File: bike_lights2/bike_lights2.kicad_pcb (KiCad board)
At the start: 2 copper layers, 36 x 18 mm, 36 parts, among them J2 LED, J3 B+, P1 USB_C_Plug_USB2.0, SW1 TL49, U1 TL431DBZ, U3 MIC2289, U4 MCP6002-xMS, U5 MCP73831-2-ADI/OT

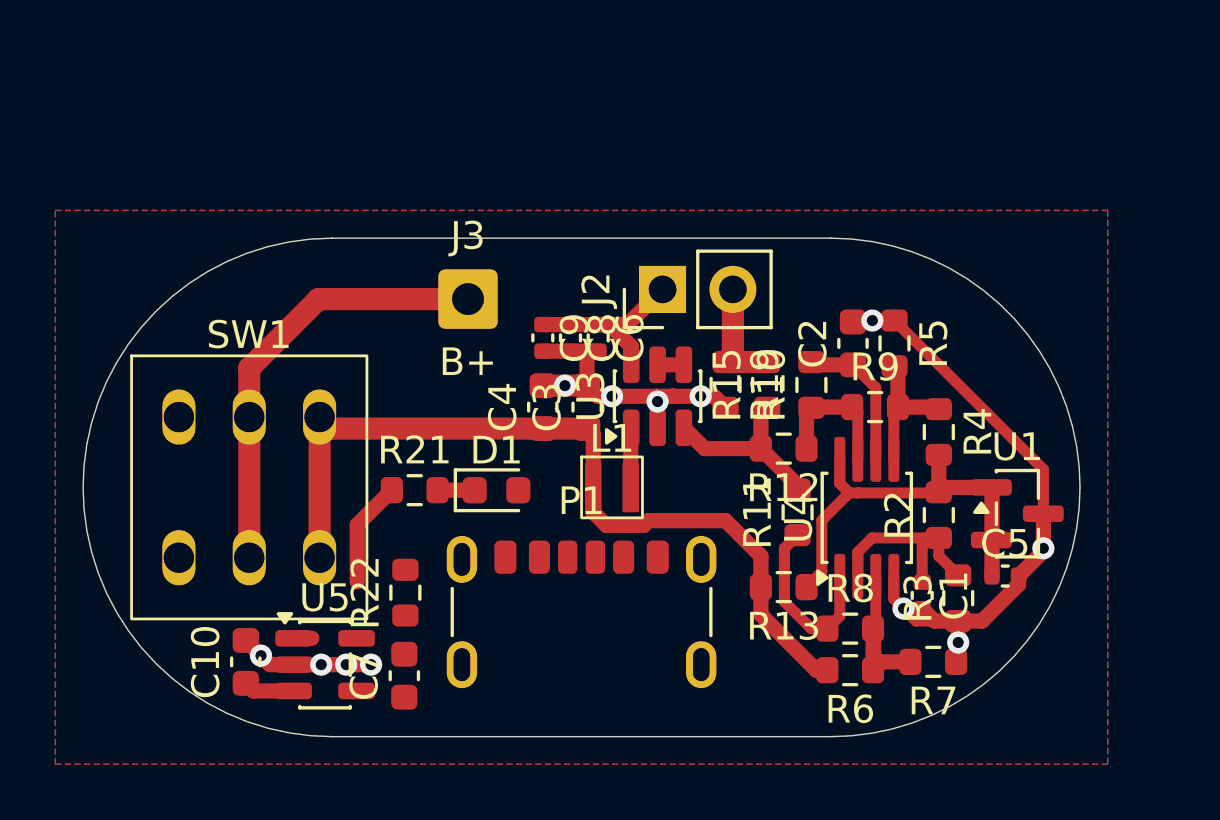
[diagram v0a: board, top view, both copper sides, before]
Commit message: a
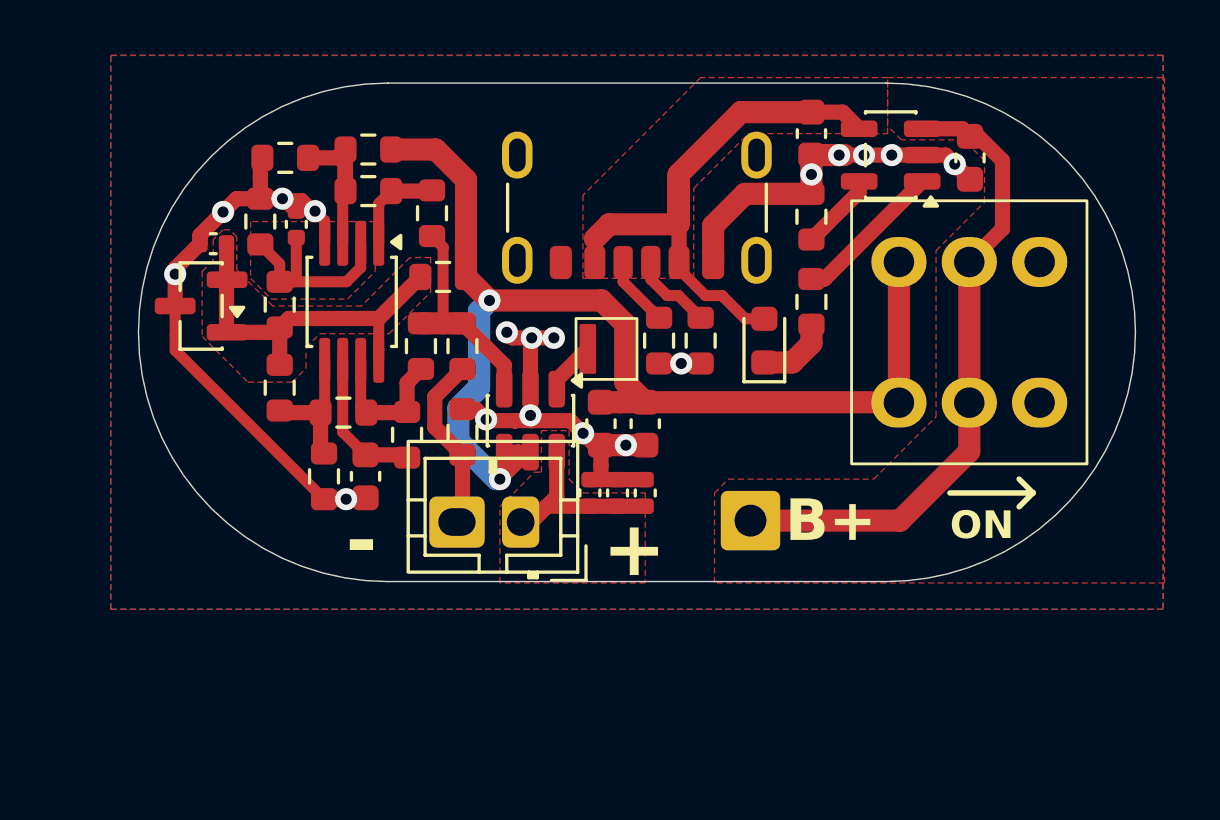
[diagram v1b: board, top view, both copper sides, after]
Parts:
- added R1: 5k1, Resistor_SMD:R_0603_1608Metric, F.Cu at (105.0, 59.5)
- added R14: 5k1, Resistor_SMD:R_0603_1608Metric, F.Cu at (106.5, 59.5)
- J2: footprint Connector_PinHeader_2.54mm:PinHeader_1x02_P2.54mm_Vertical -> footprints:JST_PH_1x02_P2.0-2.5mm_Vertical
- moved C10 31.9 mm to (116.2, 52.9), turned to -90 degrees
- moved C5 31.0 mm to (88.9, 56.0), turned to 180 degrees
- moved U1 30.4 mm to (88.5, 58.2), turned to 180 degrees
- moved R7 29.6 mm to (91.5, 52.9), turned to 0 degrees
- moved R3 28.6 mm to (90.6, 55.2), turned to -90 degrees
- moved U5 27.5 mm to (113.4, 52.8), turned to 180 degrees
- moved SW1 26.6 mm to (116.2, 59.2), turned to 180 degrees
- moved C1 26.3 mm to (91.9, 55.3), turned to 90 degrees
- moved R6 25.6 mm to (94.5, 52.6), turned to 0 degrees
- moved R2 25.0 mm to (91.3, 58.2), turned to -90 degrees
- moved C7 24.5 mm to (110.5, 52.0), turned to -90 degrees
- moved R4 23.9 mm to (91.3, 61.2), turned to 90 degrees
- moved R8 23.5 mm to (94.5, 54.1), turned to 180 degrees
- moved R5 21.2 mm to (92.9, 64.4), turned to 90 degrees
- moved U4 20.2 mm to (93.9, 58.1), turned to -90 degrees
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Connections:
- P1 pad A5: unconnected-(P1-CC-PadA5) -> /CC1
- P1 pad B5: unconnected-(P1-VCONN-PadB5) -> /CC2
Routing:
- net /Vusb: track 0.00 -> 20.7 mm
- net GND: track 39.1 -> 52.4 mm, vias 12 -> 18
- net +BATT: track 31.2 -> 44.0 mm, vias 0 -> 2
- net /Battery: track 17.6 -> 23.3 mm
- net /LowBat: track 6.63 -> 3.56 mm
- net /CC1: track 0.00 -> 2.98 mm
- net Net-(U5-PROG): track 0.00 -> 2.81 mm
- net /CC2: track 0.00 -> 2.53 mm
- net /LED-: track 4.23 -> 6.66 mm
- net Net-(D1-K): track 1.38 -> 2.66 mm
- net +2V5: track 15.2 -> 13.9 mm
- net /LED+: track 6.63 -> 7.83 mm
- net /FB: track 6.68 -> 7.82 mm
- net /CHG: track 4.49 -> 5.46 mm
- added copper zone on F.Cu, net +2V5
- added copper zone on F.Cu, net /Battery
- added copper zone on F.Cu, net /LED+
- added copper zone on F.Cu, net /Vref
- added copper zone on F.Cu, net /Vusb
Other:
- board text added: "+"
- board text added: "-"
- board text added: "Bike Lights"
- board text added: "ON"
- board text added: "revA 8/26 X.B."
